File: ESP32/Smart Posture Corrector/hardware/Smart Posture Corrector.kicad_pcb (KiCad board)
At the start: 2 copper layers, 106.5 x 93.9 mm, 64 parts, among them J1 MPU6050, J10 -5V, J11 USB_C Conn, J15 SD MODULE, J24 BSENS, J5 +IN, J6 -IN, J9 +5V, M1 Motor_DC, Q1 UMH3N, SW1 SW_Push, SW2 RESET, SW3 FLASH, U1 LM2596S-3.3V, U2 AMS1117-3.3, U3 ESP32-WROOM, U4 CH340C, Y1 12MHz

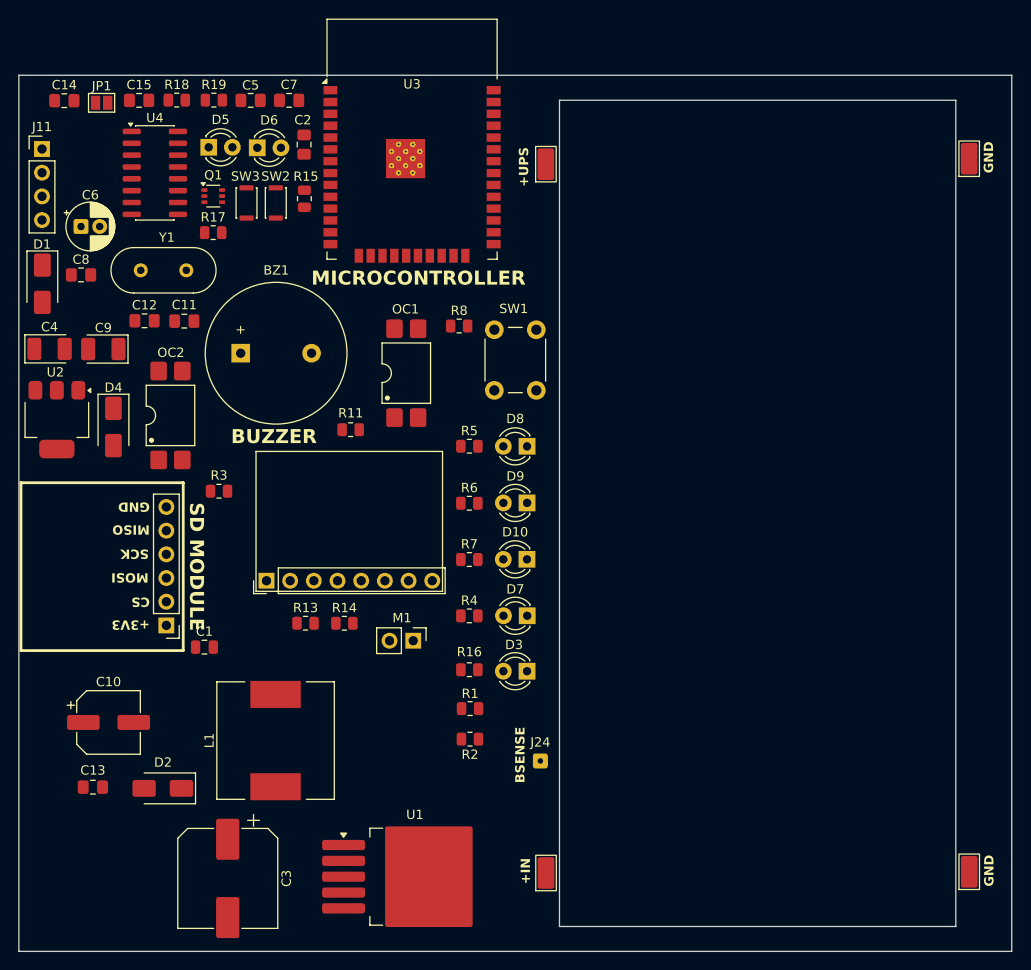
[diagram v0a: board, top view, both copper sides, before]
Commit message: Update from home
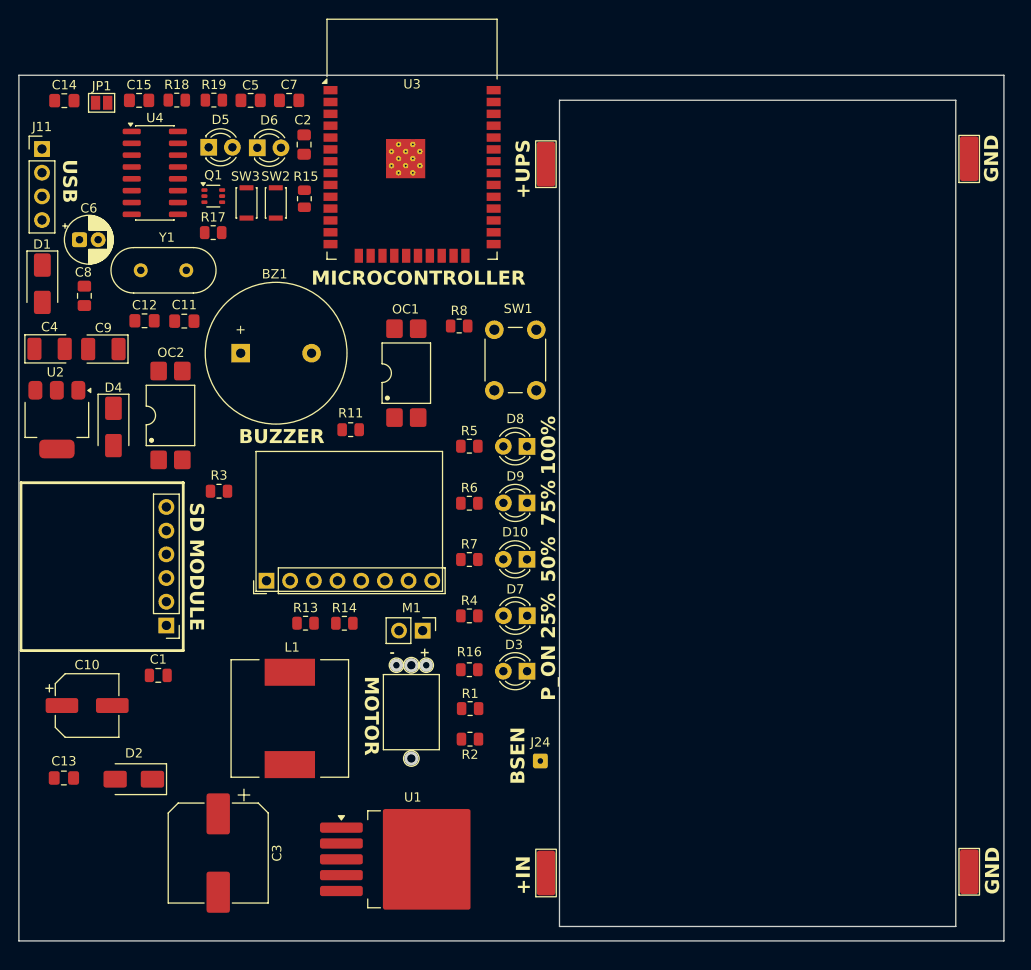
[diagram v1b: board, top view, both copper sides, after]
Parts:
- moved C1 5.81 mm to (139.0, 122.7), turned to 180 degrees
- moved D2 3.26 mm to (136.4, 133.9)
- moved C13 3.26 mm to (128.9, 133.7)
- moved C10 2.93 mm to (131.4, 126.0)
- moved C3 2.91 mm to (145.5, 141.8)
- moved L1 2.82 mm to (153.2, 127.3)
- moved C8 2.27 mm to (131.1, 82.0), turned to 90 degrees
- moved U1 1.88 mm to (166.3, 142.5)
- moved M1 1.48 mm to (167.4, 117.9)
- moved C6 1.42 mm to (130.6, 76.0)
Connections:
- M1 pad 1: VCC -> +3.3V
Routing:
- net Net-(M1--): vias 0 -> 1
- net GND: vias 0 -> 2
- net +3.3V: vias 0 -> 1
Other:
- board size 106.5 x 93.9 mm -> 105.6 x 92.8 mm
- board text added: "+"
- board text added: "+5V"
- board text added: "-"
- board text added: "100%"
- board text added: "25%"
- board text added: "50%"
- board text added: "75%"
- board text added: "AD0"
- board text added: "BSEN"
- board text added: "D+"
- board text added: "D-"
- board text added: "INT"
- board text added: "MOTOR"
- board text added: "P_ON"
- board text added: "SCL"
- board text added: "SDA"
- board text added: "USB"
- board text added: "XCL"
- board text added: "XDA"
- board text removed: "BSENSE"
